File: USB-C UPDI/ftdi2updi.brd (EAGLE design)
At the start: 33.1 x 26.6 mm, 6 parts, among them J2 61300511121

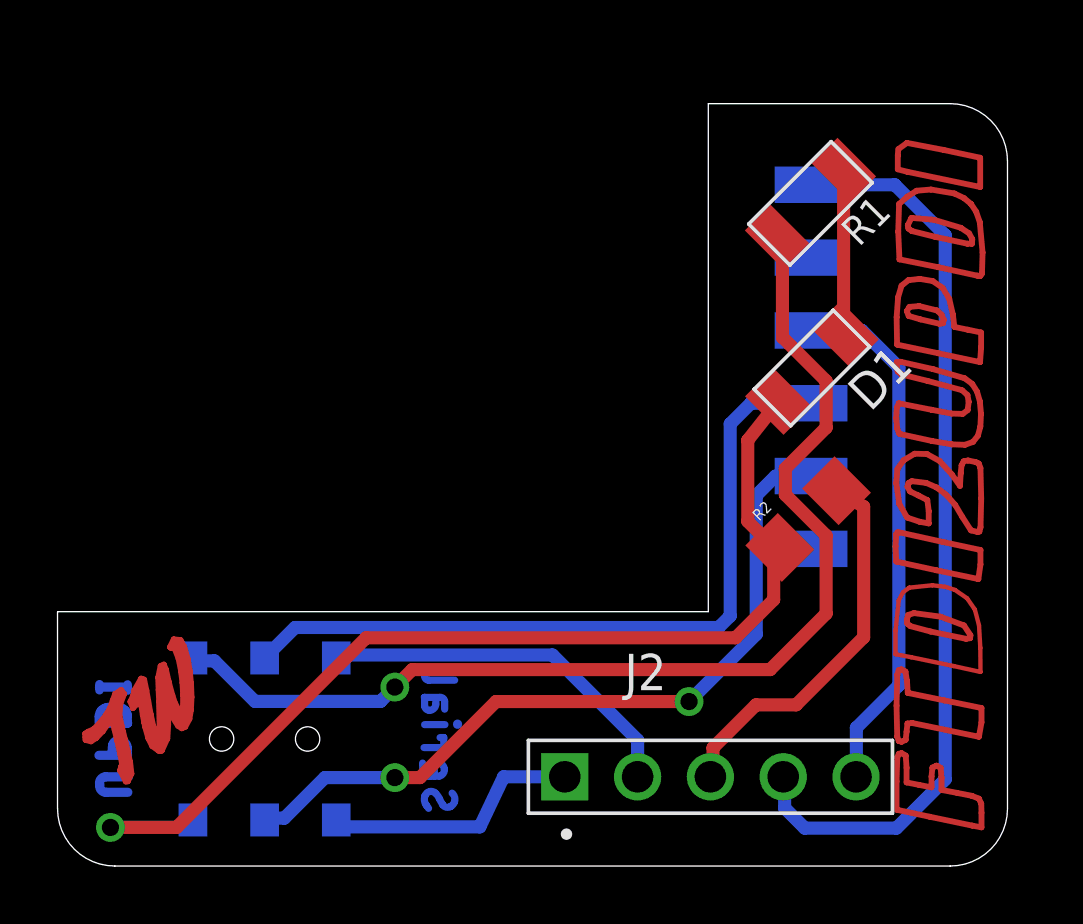
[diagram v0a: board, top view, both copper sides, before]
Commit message: updates
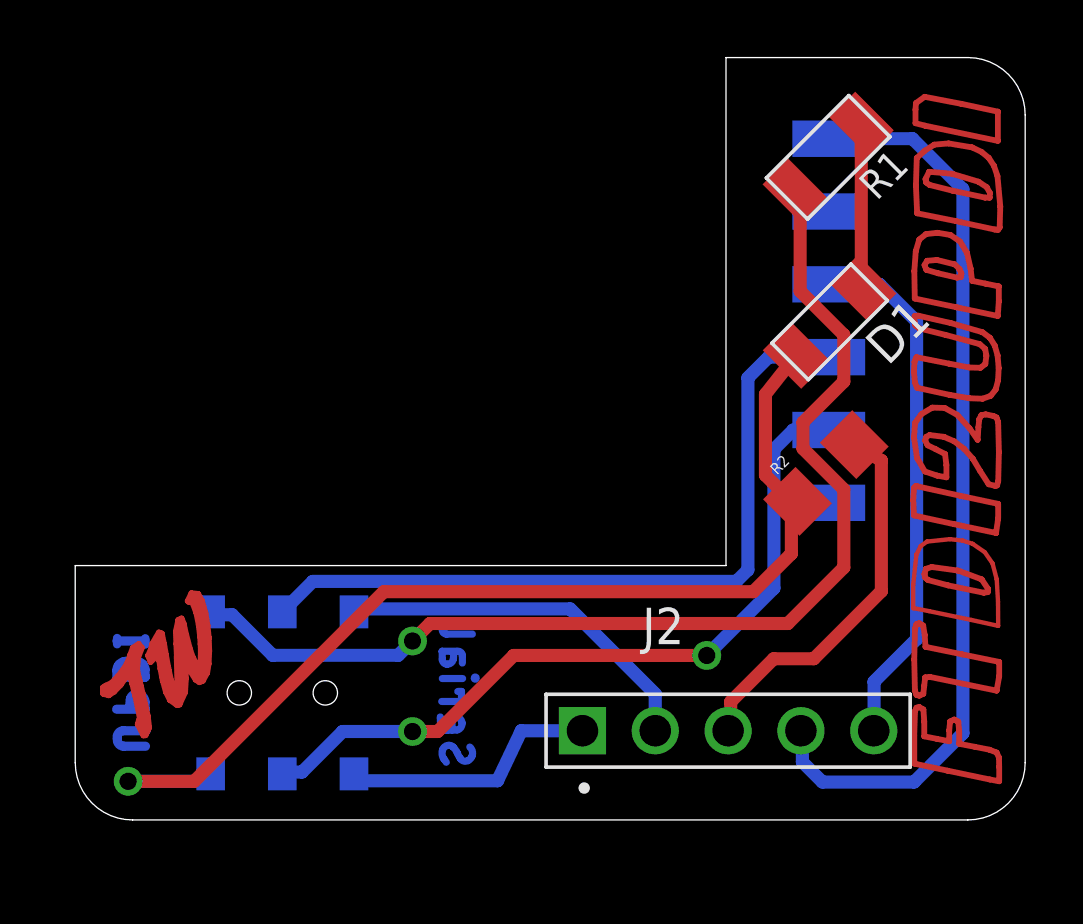
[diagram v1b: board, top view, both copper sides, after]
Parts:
- moved S1 1.72 mm to (8.84, 6.91)
- moved D1 1.72 mm to (27.9, 19.9)
- moved R1 1.72 mm to (27.9, 25.6)
- moved J2 1.72 mm to (24.4, 5.59)
- moved R2 1.72 mm to (27.8, 14.6)
- moved U$1 1.72 mm to (27.9, 19.9)
